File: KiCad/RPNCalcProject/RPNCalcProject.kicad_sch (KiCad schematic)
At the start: 78 parts, among them SW1 SW_MEC_5G, SW10 SW_MEC_5G, SW11 SW_MEC_5G, SW12 SW_MEC_5G, SW13 SW_MEC_5G, SW14 SW_MEC_5G, SW15 SW_MEC_5G, SW16 SW_MEC_5G, SW17 SW_MEC_5G, SW18 SW_MEC_5G, SW19 SW_MEC_5G, SW2 SW_MEC_5G, SW20 SW_MEC_5G, SW21 SW_MEC_5G, SW22 SW_MEC_5G, SW23 SW_MEC_5G, SW24 SW_MEC_5G, SW25 SW_MEC_5G, SW26 SW_MEC_5G, SW27 SW_MEC_5G, SW28 SW_MEC_5G, SW29 SW_MEC_5G, SW3 SW_MEC_5G, SW30 SW_MEC_5G, SW31 SW_MEC_5G, SW32 SW_MEC_5G, SW33 SW_MEC_5G, SW34 SW_MEC_5G, SW35 SW_MEC_5G, SW36 SW_MEC_5G, SW4 SW_MEC_5G, SW5 SW_MEC_5G, SW6 SW_MEC_5G, SW7 SW_MEC_5G, SW8 SW_MEC_5G, SW9 SW_MEC_5G, U1 MSP430G2553IPW20, U2 MCP23017_SO, U3 74HC595

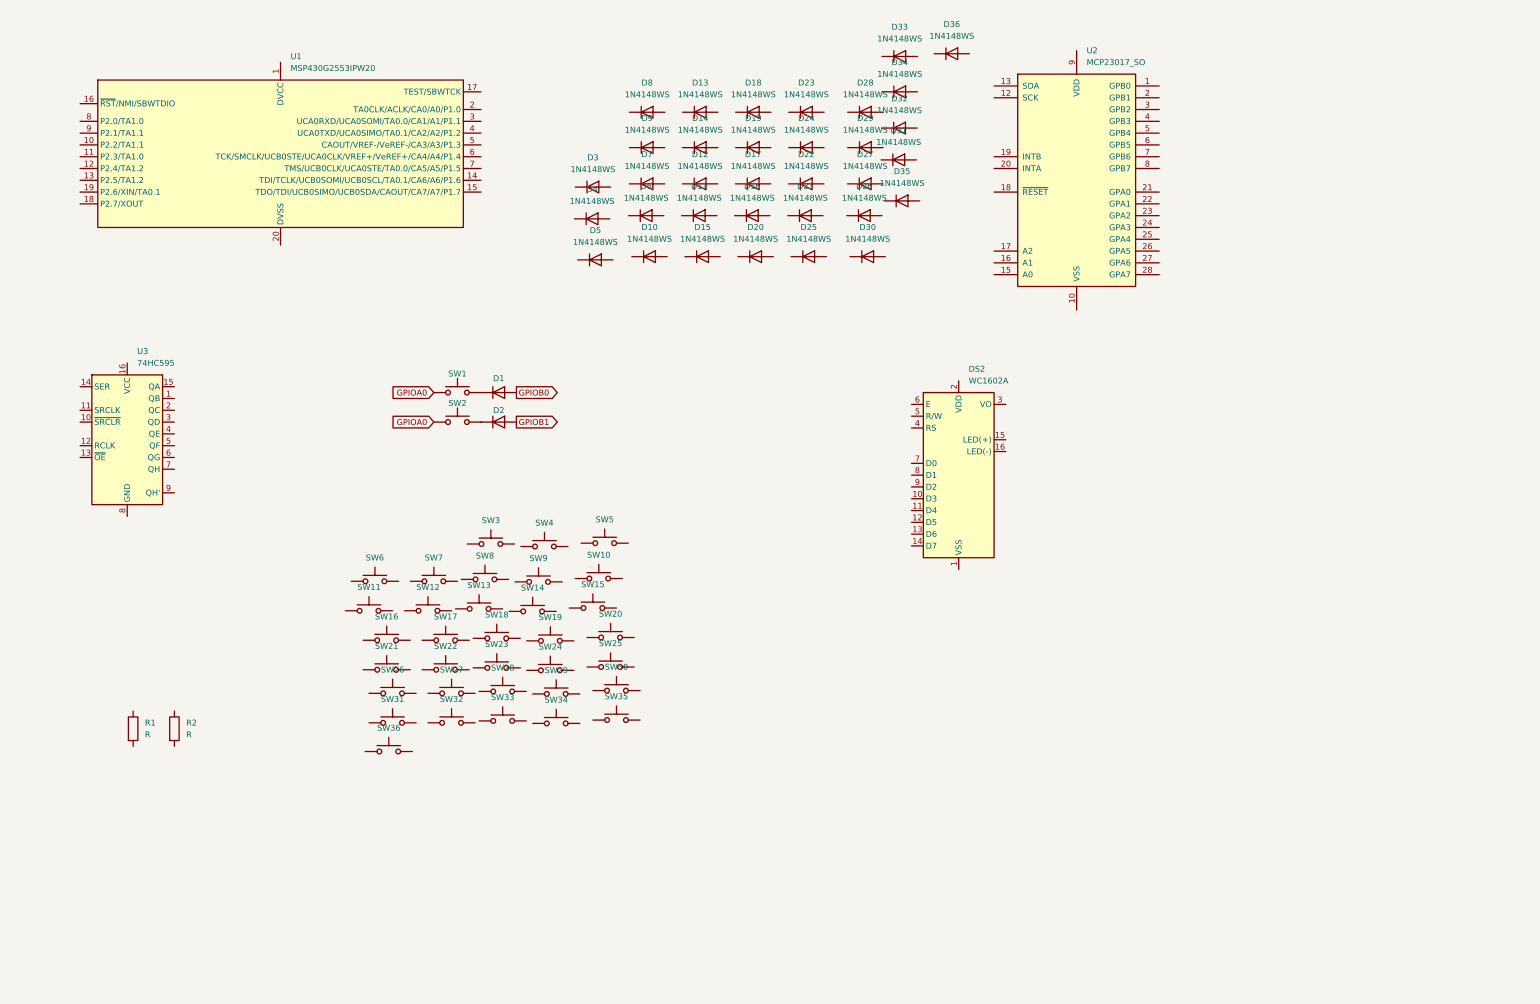
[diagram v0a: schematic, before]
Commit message: Updated kicad schematic
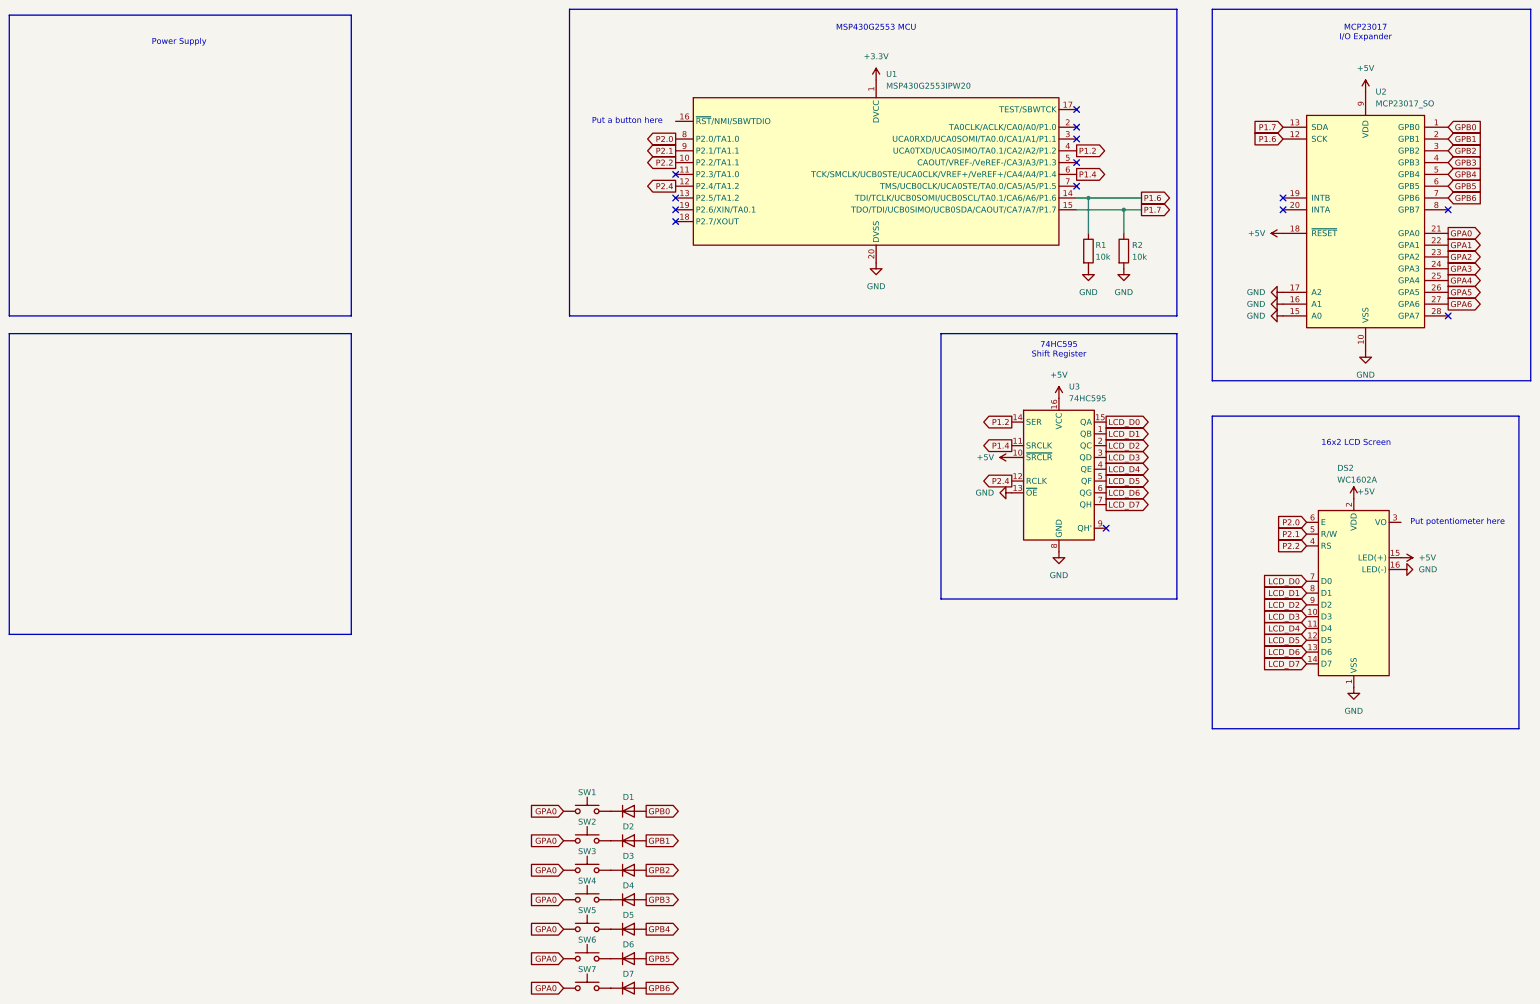
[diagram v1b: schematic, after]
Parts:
- removed D10, D11, D12, D13, D14, D15, D16, D17, D18, D19, D20, D21, D22, D23, D24, D25, D26, D27, D28, D29, D30, D31, D32, D33, D34, D35, D36, D8, D9: 1N4148WS, Diode_THT:D_DO-35_SOD27_P2.54mm_Vertical_KathodeUp, symbol Diode:1N4148WS
- removed SW10, SW11, SW12, SW13, SW14, SW15, SW16, SW17, SW18, SW19, SW20, SW21, SW22, SW23, SW24, SW25, SW26, SW27, SW28, SW29, SW30, SW31, SW32, SW33, SW34, SW35, SW36, SW8, SW9: SW_MEC_5G, Momentary Tactile Buttons:Tactile momentary button, symbol Switch:SW_MEC_5G
- R1, R2: value R -> 10k
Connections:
- net GPIOA0 is gone; now on net GPA0: SW1.1 (A), SW1.2 (A), SW2.1 (A), SW2.2 (A)
- net GPIOB0 is gone; now on net GPB0: D1.2 (A)
- net GPIOB1 is gone; now on net GPB1: D2.2 (A)
- net GND: now reaches DS2.1 (VSS)
- net GND: now also DS2.16 (LED(-)), R1.2, R2.2, U1.20 (DVSS), U2.10 (VSS), U2.15 (A0), U2.16 (A1), U2.17 (A2), U3.13 (~{OE}), U3.8 (GND)
- net LCD_D3: now reaches DS2.10 (D3)
- net LCD_D3: now also U3.3 (QD)
- net LCD_D4: now reaches DS2.11 (D4)
- net LCD_D4: now also U3.4 (QE)
- net LCD_D5: now reaches DS2.12 (D5)
- net LCD_D5: now also U3.5 (QF)
- net LCD_D6: now reaches DS2.13 (D6)
- net LCD_D6: now also U3.6 (QG)
- net LCD_D7: now reaches DS2.14 (D7)
- net LCD_D7: now also U3.7 (QH)
- net +5V: now reaches DS2.15 (LED(+))
- net +5V: now also DS2.2 (VDD), U2.18 (~{RESET}), U2.9 (VDD), U3.10 (~{SRCLR}), U3.16 (VCC)
- net P2.2: now reaches DS2.4 (RS)
- net P2.2: now also U1.10 (P2.2/TA1.1)
- net P2.1: now reaches DS2.5 (R/W)
- net P2.1: now also U1.9 (P2.1/TA1.1)
- net P2.0: now reaches DS2.6 (E)
- net P2.0: now also U1.8 (P2.0/TA1.0)
- net LCD_D0: now reaches DS2.7 (D0)
- net LCD_D0: now also U3.15 (QA)
- net LCD_D1: now reaches DS2.8 (D1)
- net LCD_D1: now also U3.1 (QB)
- net LCD_D2: now reaches DS2.9 (D2)
- net LCD_D2: now also U3.2 (QC)
- net P1.6: now reaches R1.1
- net P1.6: now also U1.14 (TDI/TCLK/UCB0SOMI/UCB0SCL/TA0.1/CA6/A6/P1.6), U2.12 (SCK)
- net GPA0: now reaches SW6.1 (A), SW6.2 (A)
- net GPA0: now also SW3.1 (A), SW3.2 (A), SW4.1 (A), SW4.2 (A), SW5.1 (A), SW5.2 (A), SW7.1 (A), SW7.2 (A), U2.21 (GPA0)
- net at SW6.3 (B), SW6.4 (B): now also D6.1 (K)
- net P1.4: now reaches U3.11 (SRCLK)
- net P1.4: now also U1.6 (TCK/SMCLK/UCB0STE/UCA0CLK/VREF+/VeREF+/CA4/A4/P1.4)
- net P2.4: now reaches U3.12 (RCLK)
- net P2.4: now also U1.12 (P2.4/TA1.2)
- net P1.2: now reaches U3.14 (SER)
- net P1.2: now also U1.4 (UCA0TXD/UCA0SIMO/TA0.1/CA2/A2/P1.2)
- net at SW7.3 (B), SW7.4 (B): now also D7.1 (K)
- net at SW5.3 (B), SW5.4 (B): now also D5.1 (K)
- net +3.3V: now reaches U1.1 (DVCC)
- net P1.7: now reaches U1.15 (TDO/TDI/UCB0SIMO/UCB0SDA/CAOUT/CA7/A7/P1.7)
- net P1.7: now also R2.1, U2.13 (SDA)
- net at D3.1 (K): now also SW3.3 (B), SW3.4 (B)
- net GPB2: now reaches D3.2 (A)
- net GPB2: now also U2.3 (GPB2)
- net GPB4: now reaches D5.2 (A)
- net GPB4: now also U2.5 (GPB4)
- net at SW4.3 (B), SW4.4 (B): now also D4.1 (K)
- net GPB0: now reaches U2.1 (GPB0)
- net GPB1: now reaches U2.2 (GPB1)
- net GPA1: now reaches U2.22 (GPA1)
- net GPA2: now reaches U2.23 (GPA2)
- net GPA3: now reaches U2.24 (GPA3)
- net GPA4: now reaches U2.25 (GPA4)
- net GPA5: now reaches U2.26 (GPA5)
- net GPA6: now reaches U2.27 (GPA6)
- net GPB3: now reaches U2.4 (GPB3)
- net GPB3: now also D4.2 (A)
- net GPB5: now reaches U2.6 (GPB5)
- net GPB5: now also D6.2 (A)
- net GPB6: now reaches U2.7 (GPB6)
- net GPB6: now also D7.2 (A)
- no-connect marks 0 -> 14
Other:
- note added: "16x2 LCD Screen"
- note added: "74HC595 Shift Register"
- note added: "MCP23017 I/O Expander"
- note added: "MSP430G2553 MCU"
- note added: "Power Supply"
- note added: "Put a button here"
- note added: "Put potentiometer here"
- moved on the sheet: D1, DS2, R1, R2, SW1, U1, U2, U3
